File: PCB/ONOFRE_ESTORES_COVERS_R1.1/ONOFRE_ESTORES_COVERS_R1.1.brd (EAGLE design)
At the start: 44.1 x 43.8 mm, 30 parts, among them J1 9PIN 2.54MM, J3Y S8050, J7 8p, K1 G5Q-1-DC12, K2 G5Q-1-DC12, U2 esp12

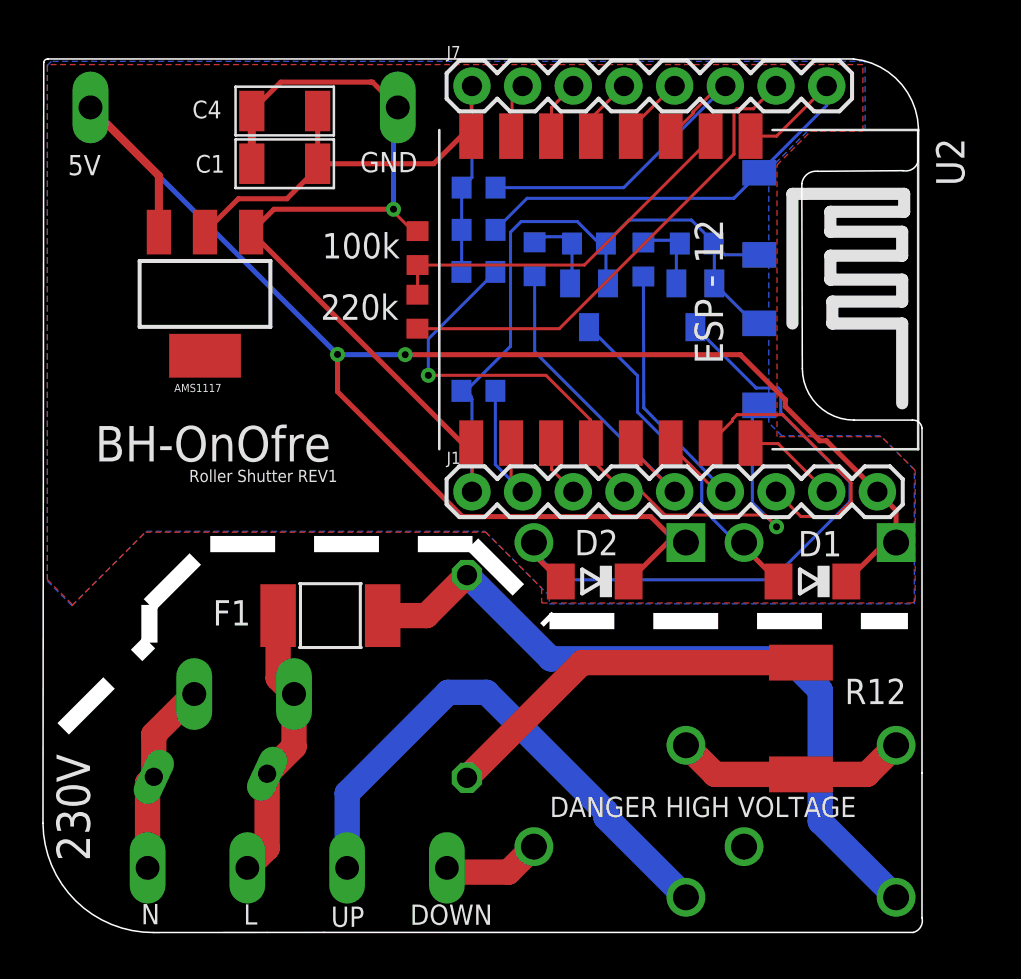
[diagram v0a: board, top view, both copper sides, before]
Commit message: estores
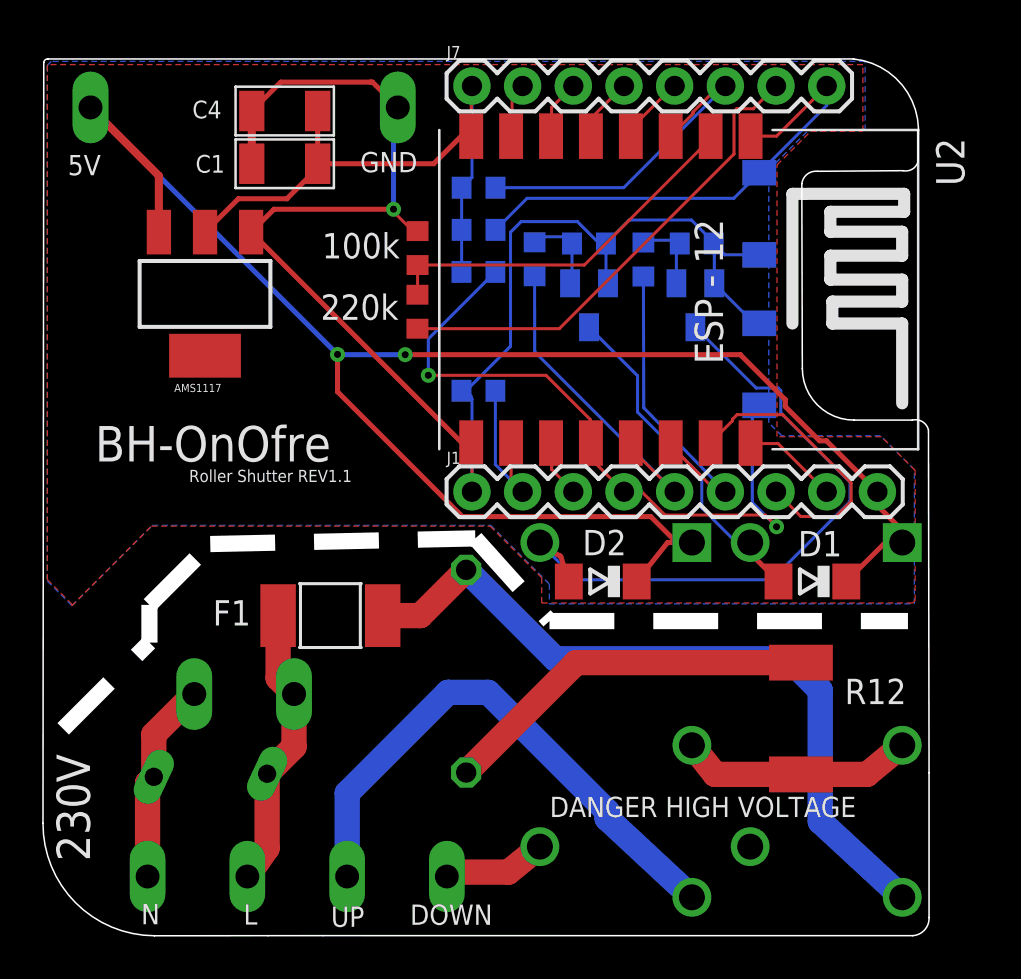
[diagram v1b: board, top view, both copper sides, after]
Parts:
- moved X1 0.43 mm to (13.4, 4.08)
- moved D2 0.40 mm to (28.7, 20.1)
- moved K1 0.31 mm to (39.8, 13.1)
- moved K2 0.30 mm to (29.2, 13.1)
- moved C6 0.27 mm to (21.9, 15.6)
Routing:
- net VCC: track 87.7 -> 88.4 mm
- net LINE_UP_OUT: track 27.2 -> 27.9 mm
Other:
- board size 44.1 x 43.8 mm -> 44.4 x 43.9 mm
- board text added: "Roller Shutter REV1.1"
- board text removed: "Roller Shutter REV1"
